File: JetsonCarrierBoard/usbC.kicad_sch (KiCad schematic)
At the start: 42 parts, among them J4 USB_C_Receptacle, U6 TPD6S300A, U7 HD3SS460

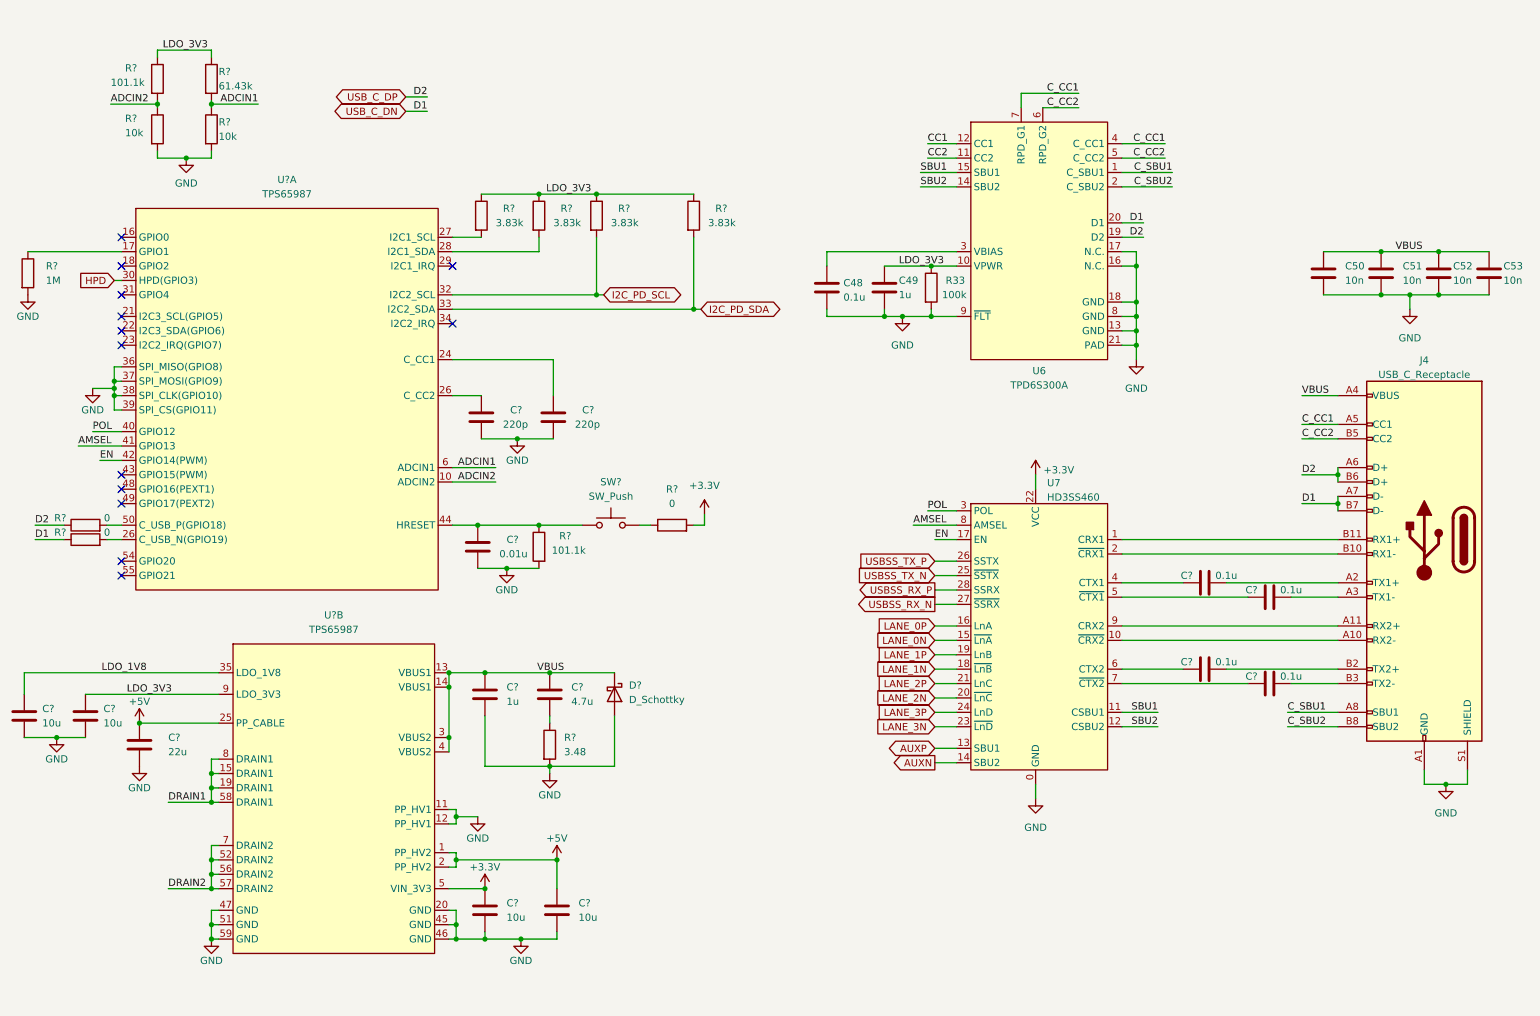
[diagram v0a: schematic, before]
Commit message: USB-C Changes
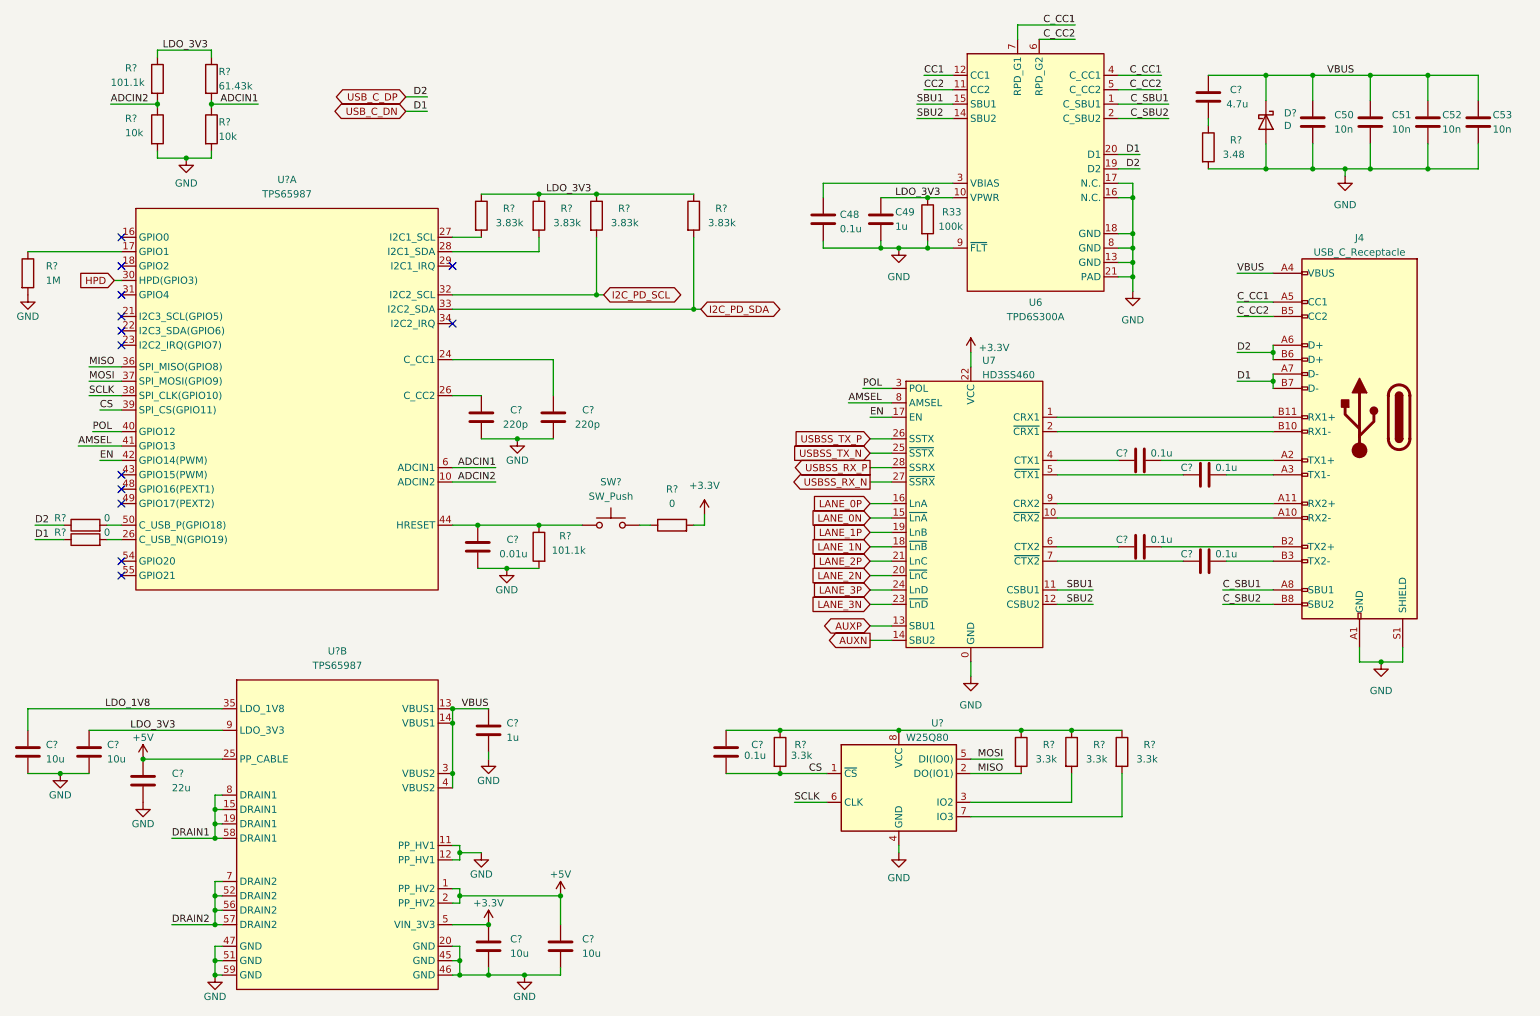
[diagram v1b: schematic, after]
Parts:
- removed C?: 4.7u, symbol Device:C
- removed D?: D_Schottky, symbol Device:D_Schottky
- removed R?: 3.48, symbol Device:R
- added C?: 4.7u, symbol Device:C
- added C?: 0.1u, symbol Device:C
- added D?: D, symbol Device:D_Schottky
- added R? (x4): 3.3k, symbol Device:R
- added R?: 3.48, symbol Device:R
- added U?: W25Q80, Package_SO:SOIC-8_5.23x5.23mm_P1.27mm, symbol Memory_Flash:W25Q128JVS
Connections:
- net GND: now also D?.2 (A), R?.2, U?.4 (GND); no longer U?.36 (SPI_MISO(GPIO8)), U?.37 (SPI_MOSI(GPIO9)), U?.38 (SPI_CLK(GPIO10)), U?.39 (SPI_CS(GPIO11))
- net VBUS: now also C?.2, D?.1 (K)
- new net: C?.2, R?.1, R?.1, R?.1, R?.1, U?.8 (VCC)
- new net: C?.1, R?.1
- new net: R?.2, U?.3 (IO2)
- new net: R?.2, U?.7 (IO3)
- new net CS: C?.1, R?.2, U?.1 (~{CS}), U?.39 (SPI_CS(GPIO11))
- new net MISO: R?.2, U?.2 (DO(IO1)), U?.36 (SPI_MISO(GPIO8))
- new net MOSI: U?.37 (SPI_MOSI(GPIO9)), U?.5 (DI(IO0))
- new net SCLK: U?.38 (SPI_CLK(GPIO10)), U?.6 (CLK)
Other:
- moved on the sheet: C48, C49, C50, C51, C52, C53, C?, J4, R33, U6, U7, U?B
